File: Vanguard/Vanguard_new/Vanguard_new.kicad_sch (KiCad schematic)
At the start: 72 parts, among them J1 USB_C, J2 Conn_02x03_Pin, J3 Micro_SD_Card_Det1, J4 STARBOARD_SERVO, J5 PORTSIDE_SERVO, J6 LIPO_in, Q1 BSS138, Q2 BSS138, Q3 BSS138, Q4 BSS138, U1 ATSAMD11D14A-M, U2 ATmega4809-A, U3 AT25DF641A-SH-T, U4 AP2112K-3.3, U5 MPM3610AGQV-P, U6 BNO086, U7 TXB0104D, U8 TPS61092, Y1 32.768kHz

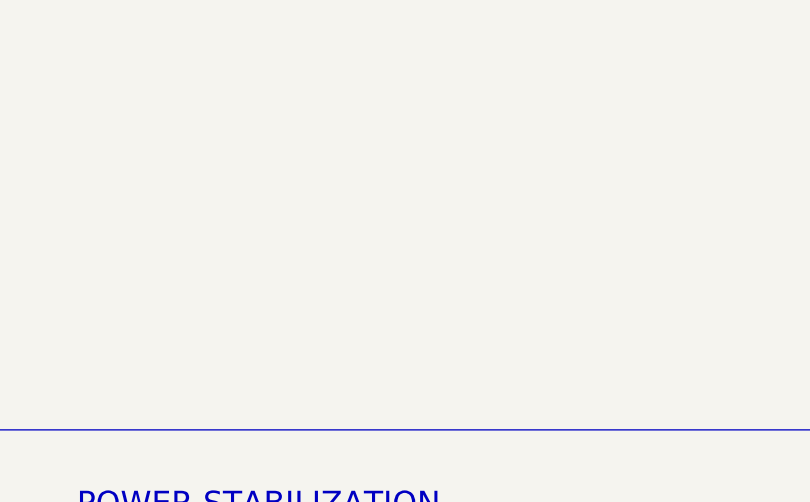
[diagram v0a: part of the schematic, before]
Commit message: pcb work
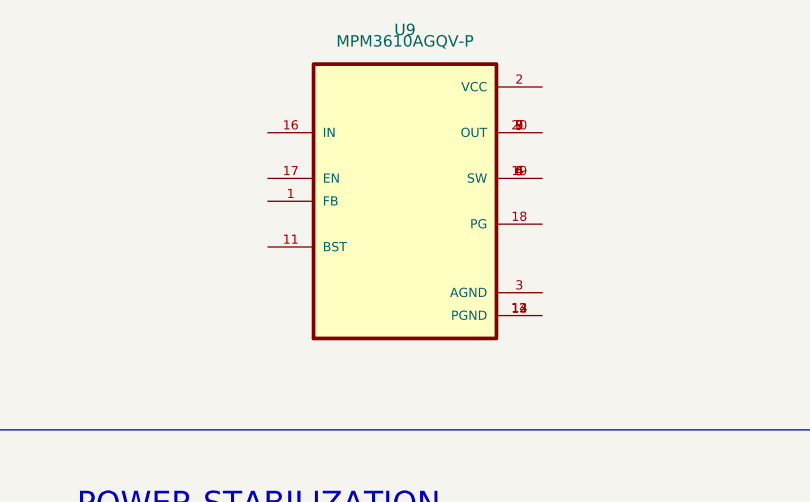
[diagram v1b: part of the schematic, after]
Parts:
- added U9: MPM3610AGQV-P, MPM3610AGQV-P:CONV_MPM3620AGQV-P, symbol MPM3610AGQV-P:MPM3610AGQV-P
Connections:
- new net: U9.12 (PGND), U9.13 (PGND), U9.14 (PGND)
- new net: U9.19 (SW), U9.4 (SW), U9.5 (SW), U9.6 (SW)
- new net: U9.20 (OUT), U9.7 (OUT), U9.8 (OUT), U9.9 (OUT)
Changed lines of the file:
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@@
+	)
+	(symbol
+		(lib_name "MPM3610AGQV-P_1")
+		(lib_id "MPM3610AGQV-P:MPM3610AGQV-P")
+		(at 317.5 -11.43 0)
+		(unit 1)
+		(exclude_from_sim no)
+		(in_bom yes)
+		(on_board yes)
+		(dnp no)
+		(fields_autoplaced yes)
+		(property "Reference" "U9"
+			(at 317.5 -30.48 0)
+			(effects
+				(font
+					(size 1.27 1.27)
+				)
+			)
+		)
+		(property "Value" "MPM3610AGQV-P"
+			(at 317.5 -29.21 0)
+			(effects
+				(font
+					(size 1.27 1.27)
+				)
+			)
+		)
+		(property "Footprint" "MPM3610AGQV-P:CONV_MPM3620AGQV-P"
+			(at 317.5 -11.43 0)
+			(effects
+				(font
+					(size 1.27 1.27)
+				)
+				(justify bottom)
+				(hide yes)
+			)
+		)
+		(property "Datasheet" ""
+			(at 317.5 -11.43 0)
+			(effects
+				(font
+					(size 1.27 1.27)
+				)
+				(hide yes)
+			)
+		)
+		(property "Description" ""
+			(at 317.5 -11.43 0)
+			(effects
+				(font
+					(size 1.27 1.27)
+				)
+				(hide yes)
+			)
+		)
+		(property "MF" "Monolithic Power"
+			(at 317.5 -11.43 0)
+			(effects
+				(font
+					(size 1.27 1.27)
+				)
+				(justify bottom)
+				(hide yes)
+			)
+		)
+		(property "DESCRIPTION" "MPM3610A Series 21 V 1.2 A Adj. SMT Synchronous Step-Down Converter - QFN-20"
+			(at 317.5 -11.43 0)
+			(effects
+				(font
+					(size 1.27 1.27)
+				)
+				(justify bottom)
+				(hide yes)
+			)
+		)
+		(property "PACKAGE" "QFN-20 Monolithic Power Systems"
+			(at 317.5 -11.43 0)
+			(effects
+				(font
+					(size 1.27 1.27)
+				)
+				(justify bottom)
+				(hide yes)
+			)
+		)
+		(property "PRICE" "2.62 USD"
+			(at 317.5 -11.43 0)
+			(effects
+				(font
+					(size 1.27 1.27)
+				)
+				(justify bottom)
+				(hide yes)
+			)
+		)
+		(property "Package" "QFN-20 MPS"
+			(at 317.5 -11.43 0)
+			(effects
+				(font
+					(size 1.27 1.27)
+				)
+				(justify bottom)
+				(hide yes)
+			)
+		)
+		(property "Check_prices" "https://www.snapeda.com/parts/MPM3610AGQV-P/Monolithic+Power+Systems+Inc./view-part/?ref=eda"
+			(at 317.5 -11.43 0)
+			(effects
+				(font
+					(size 1.27 1.27)
+				)
+				(justify bottom)
+				(hide yes)
+			)
+		)
+		(property "STANDARD" "Manufacturer recommendation"
+			(at 317.5 -11.43 0)
+			(effects
+				(font
+					(size 1.27 1.27)
+				)
+				(justify bottom)
+				(hide yes)
+			)
+		)
+		(property "PARTREV" "1.0"
+			(at 317.5 -11.43 0)
+			(effects
+				(font
+					(size 1.27 1.27)
+				)
+				(justify bottom)
+				(hide yes)
+			)
+		)
+		(property "SnapEDA_Link" "https://www.snapeda.com/parts/MPM3610AGQV-P/Monolithic+Power+Systems+Inc./view-part/?ref=snap"
+			(at 317.5 -11.43 0)
+			(effects
+				(font
+					(size 1.27 1.27)
+				)
+				(justify bottom)
+				(hide yes)
+			)
+		)
+		(property "MP" "MPM3610AGQV-P"
+			(at 317.5 -11.43 0)
+			(effects
+				(font
+					(size 1.27 1.27)
+				)
+				(justify bottom)
+				(hide yes)
+			)
+		)
+		(property "Price" "None"
+			(at 317.5 -11.43 0)
+			(effects
+				(font
+					(size 1.27 1.27)
+				)
+				(justify bottom)
+				(hide yes)
+			)
+		)
+		(property "Availability" "In Stock"
+			(at 317.5 -11.43 0)
+			(effects
+				(font
+					(size 1.27 1.27)
+				)
+				(justify bottom)
+				(hide yes)
+			)
+		)
+		(property "AVAILABILITY" "Bad"
+			(at 317.5 -11.43 0)
+			(effects
+				(font
+					(size 1.27 1.27)
+				)
+				(justify bottom)
+				(hide yes)
+			)
+		)
+		(property "Description_1" "\nNon-Isolated PoL Module DC DC Converter 1 Output 0.8 ~ 18.48V - - - 1.2A 4.5V - 21V Input\n"
+			(at 317.5 -11.43 0)
+			(effects
+				(font
+					(size 1.27 1.27)
+				)
+				(justify bottom)
+				(hide yes)
+			)
+		)
+		(pin "4"
+		)
+		(pin "9"
+		)
+		(pin "8"
+		)
+		(pin "2"
+		)
+		(pin "5"
+		)
+		(pin "6"
+		)
+		(pin "3"
+		)
+		(pin "1"
+		)
+		(pin "13"
+		)
+		(pin "12"
+		)
+		(pin "14"
+		)
+		(pin "11"
+		)
+		(pin "7"
+		)
+		(pin "19"
+		)
+		(pin "16"
+		)
+		(pin "20"
+		)
+		(pin "18"
+		)
+		(pin "17"
+		)
+		(instances
+			(project ""
+				(path "/972fbf12-2dcd-4fdf-b1c9-8a2880c46640"
+					(reference "U9")
+					(unit 1)
+				)
+			)
+		)
 	)
 	(symbol

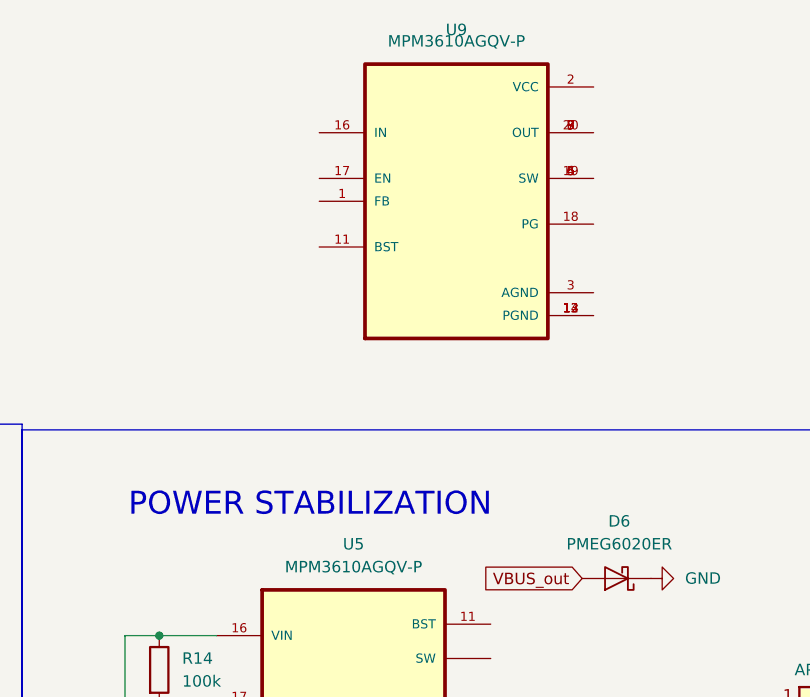
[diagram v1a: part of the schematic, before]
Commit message: just in case push
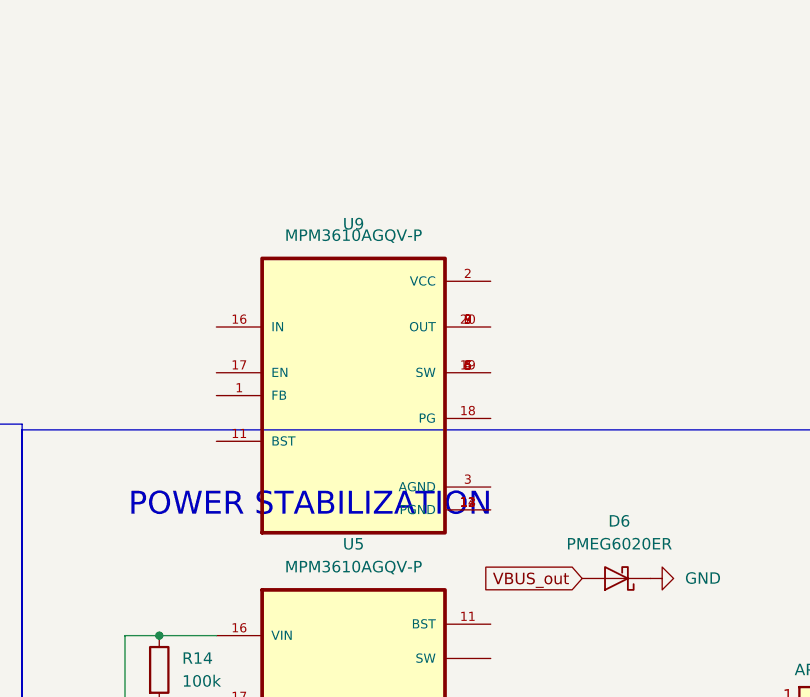
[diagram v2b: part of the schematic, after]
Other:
- moved on the sheet: U9
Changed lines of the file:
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@@
 		(lib_name "MPM3610AGQV-P_1")
 		(lib_id "MPM3610AGQV-P:MPM3610AGQV-P")
-		(at 317.5 -11.43 0)
+		(at 306.07 10.16 0)
 		(unit 1)
 		(exclude_from_sim no)
@@
 		(fields_autoplaced yes)
 		(property "Reference" "U9"
-			(at 317.5 -30.48 0)
+			(at 306.07 -8.89 0)
 			(effects
 				(font
@@
 		)
 		(property "Value" "MPM3610AGQV-P"
-			(at 317.5 -29.21 0)
+			(at 306.07 -7.62 0)
 			(effects
 				(font
@@
 		)
 		(property "Footprint" "MPM3610AGQV-P:CONV_MPM3620AGQV-P"
-			(at 317.5 -11.43 0)
+			(at 306.07 10.16 0)
 			(effects
 				(font
@@
 		)
 		(property "Datasheet" ""
-			(at 317.5 -11.43 0)
+			(at 306.07 10.16 0)
 			(effects
 				(font
@@
 		)
 		(property "Description" ""
-			(at 317.5 -11.43 0)
+			(at 306.07 10.16 0)
 			(effects
 				(font
@@
 		)
 		(property "MF" "Monolithic Power"
-			(at 317.5 -11.43 0)
+			(at 306.07 10.16 0)
 			(effects
 				(font
@@
 		)
 		(property "DESCRIPTION" "MPM3610A Series 21 V 1.2 A Adj. SMT Synchronous Step-Down Converter - QFN-20"
-			(at 317.5 -11.43 0)
+			(at 306.07 10.16 0)
 			(effects
 				(font
@@
 		)
 		(property "PACKAGE" "QFN-20 Monolithic Power Systems"
-			(at 317.5 -11.43 0)
+			(at 306.07 10.16 0)
 			(effects
 				(font
@@
 		)
 		(property "PRICE" "2.62 USD"
-			(at 317.5 -11.43 0)
+			(at 306.07 10.16 0)
 			(effects
 				(font
@@
 		)
 		(property "Package" "QFN-20 MPS"
-			(at 317.5 -11.43 0)
+			(at 306.07 10.16 0)
 			(effects
 				(font
@@
 		)
 		(property "Check_prices" "https://www.snapeda.com/parts/MPM3610AGQV-P/Monolithic+Power+Systems+Inc./view-part/?ref=eda"
-			(at 317.5 -11.43 0)
+			(at 306.07 10.16 0)
 			(effects
 				(font
@@
 		)
 		(property "STANDARD" "Manufacturer recommendation"
-			(at 317.5 -11.43 0)
+			(at 306.07 10.16 0)
 			(effects
 				(font
@@
 		)
 		(property "PARTREV" "1.0"
-			(at 317.5 -11.43 0)
+			(at 306.07 10.16 0)
 			(effects
 				(font
@@
 		)
 		(property "SnapEDA_Link" "https://www.snapeda.com/parts/MPM3610AGQV-P/Monolithic+Power+Systems+Inc./view-part/?ref=snap"
-			(at 317.5 -11.43 0)
+			(at 306.07 10.16 0)
 			(effects
 				(font
@@
 		)
 		(property "MP" "MPM3610AGQV-P"
-			(at 317.5 -11.43 0)
+			(at 306.07 10.16 0)
 			(effects
 				(font
@@
 		)
 		(property "Price" "None"
-			(at 317.5 -11.43 0)
+			(at 306.07 10.16 0)
 			(effects
 				(font
@@
 		)
 		(property "Availability" "In Stock"
-			(at 317.5 -11.43 0)
+			(at 306.07 10.16 0)
 			(effects
 				(font
@@
 		)
 		(property "AVAILABILITY" "Bad"
-			(at 317.5 -11.43 0)
+			(at 306.07 10.16 0)
 			(effects
 				(font
@@
 		)
 		(property "Description_1" "\nNon-Isolated PoL Module DC DC Converter 1 Output 0.8 ~ 18.48V - - - 1.2A 4.5V - 21V Input\n"
-			(at 317.5 -11.43 0)
+			(at 306.07 10.16 0)
 			(effects
 				(font

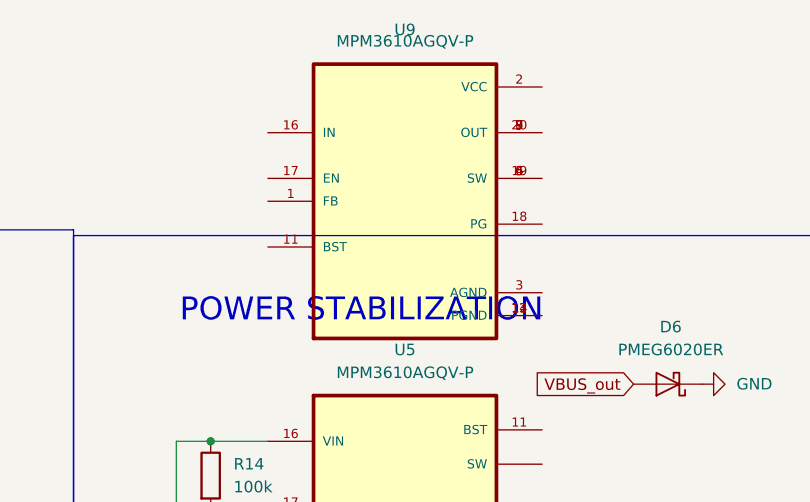
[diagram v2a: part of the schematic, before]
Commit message: usb input almost done
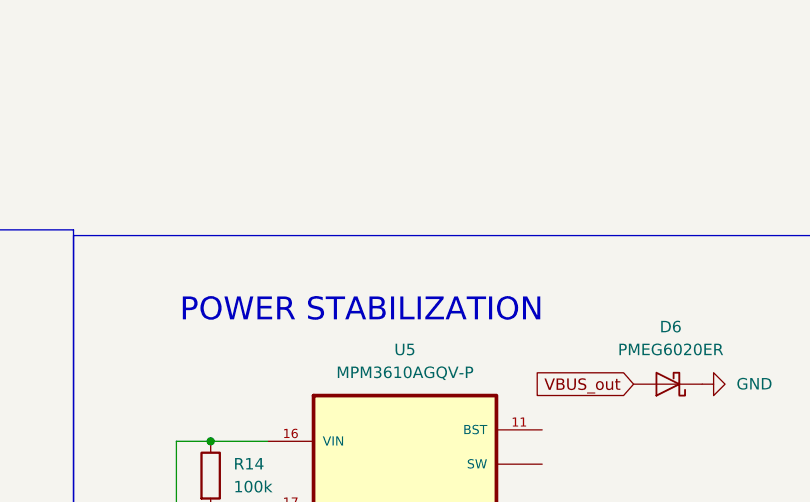
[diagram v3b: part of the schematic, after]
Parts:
- removed U9: MPM3610AGQV-P, MPM3610AGQV-P:CONV_MPM3620AGQV-P, symbol MPM3610AGQV-P:MPM3610AGQV-P
- J2: footprint Connector_PinHeader_2.54mm:PinHeader_1x03_P2.54mm_Vertical -> Connector_PinHeader_2.54mm:PinHeader_2x03_P2.54mm_Vertical
- J6: footprint CONN2_2601-1102_WAG -> Wago-2601-1102:CONN2_2601-1102_WAG
